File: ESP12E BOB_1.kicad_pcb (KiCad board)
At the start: 2 copper layers, 39.1 x 54.9 mm, 24 parts, among them M1 ESP-12E, P1 CONN_01X07, P2 CONN_01X13, P3 CONN_01X13, P4 CONN_01X01, P5 CONN_01X01, P6 CONN_01X01, P7 CONN_01X01, Q1 BSS138, Q2 BSS138, SW1 SW_PUSH, U1 1117-3.3

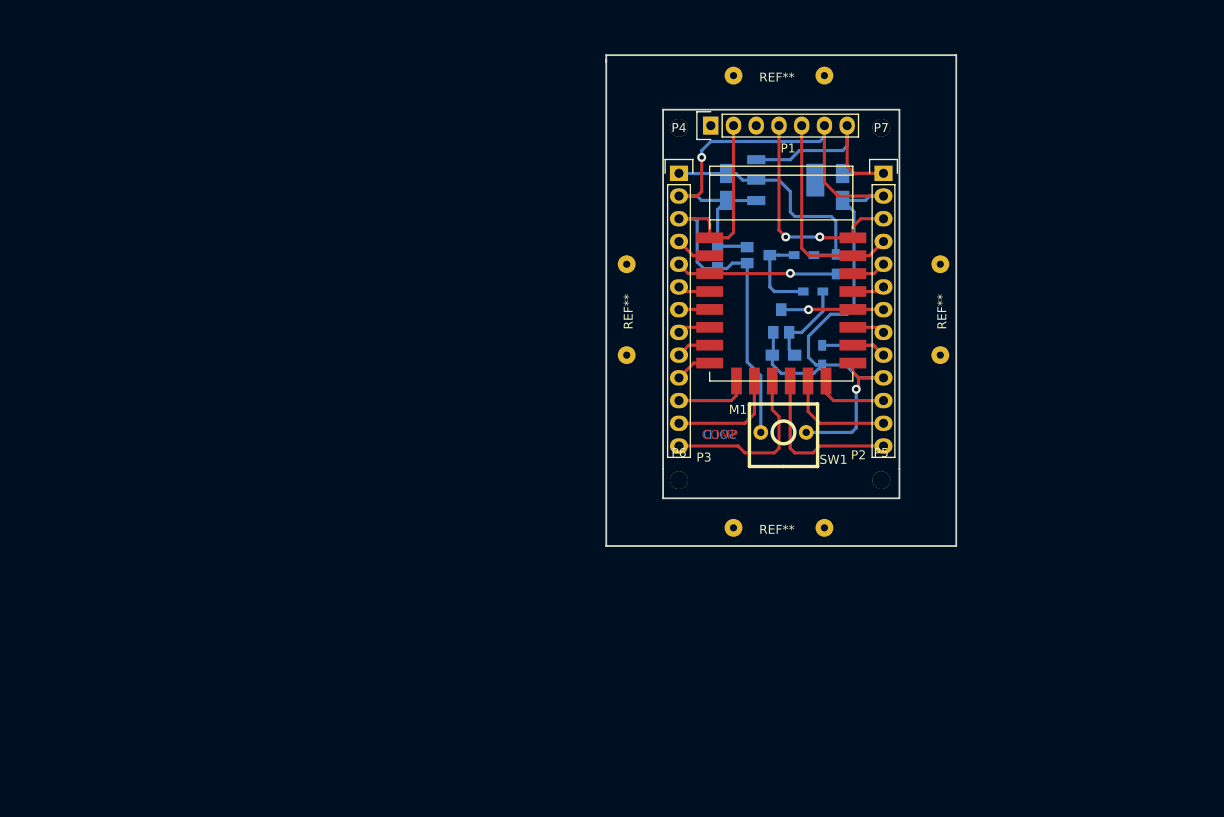
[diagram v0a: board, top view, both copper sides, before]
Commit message: ADDED FILES
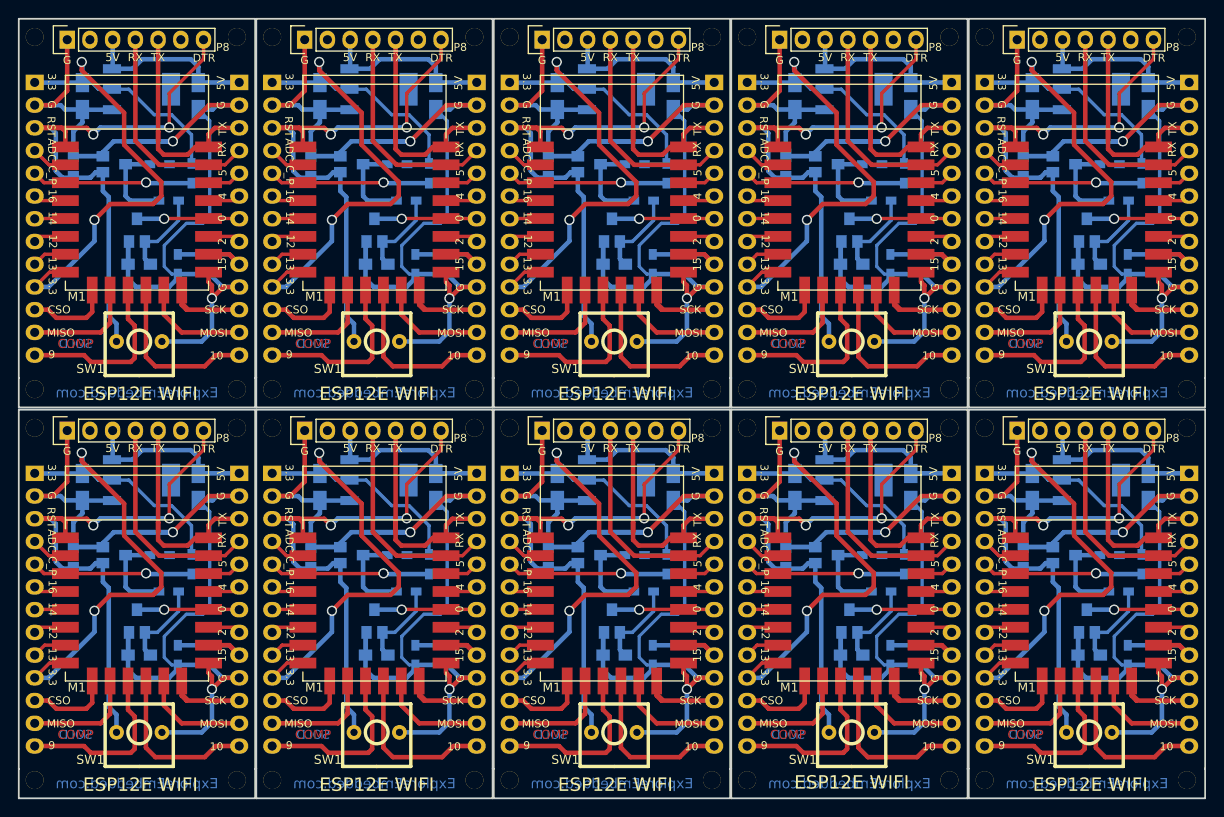
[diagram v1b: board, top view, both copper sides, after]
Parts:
- removed P1: CONN_01X07, Pin_Headers:Pin_Header_Straight_1x07
- removed the P2 at (137.2, 48.3)
- removed REF** (x4): WireConnection_0-8mmDrill, Wire_Connections_Bridges:WireConnection_0-8mmDrill
- added C1: 0.1u, Capacitors_SMD:C_0805_HandSoldering, B.Cu at (152.8, 91.2)
- added C1: 0.1u, Capacitors_SMD:C_0805_HandSoldering, B.Cu at (126.2, 91.2)
- added C1: 0.1u, Capacitors_SMD:C_0805_HandSoldering, B.Cu at (99.7, 91.2)
- added C1: 0.1u, Capacitors_SMD:C_0805_HandSoldering, B.Cu at (73.2, 91.2)
- added C1: 0.1u, Capacitors_SMD:C_0805_HandSoldering, B.Cu at (46.6, 91.2)
- added C1: 0.1u, Capacitors_SMD:C_0805_HandSoldering, B.Cu at (152.8, 47.5)
- added C1: 0.1u, Capacitors_SMD:C_0805_HandSoldering, B.Cu at (126.2, 47.5)
- added C1: 0.1u, Capacitors_SMD:C_0805_HandSoldering, B.Cu at (99.7, 47.5)
- added C1: 0.1u, Capacitors_SMD:C_0805_HandSoldering, B.Cu at (73.2, 47.5)
- added C2: 2u2, Capacitors_SMD:C_0805_HandSoldering, B.Cu at (160.1, 102.1)
- added C2: 2u2, Capacitors_SMD:C_0805_HandSoldering, B.Cu at (133.6, 102.1)
- added C2: 2u2, Capacitors_SMD:C_0805_HandSoldering, B.Cu at (107.1, 102.1)
- added C2: 2u2, Capacitors_SMD:C_0805_HandSoldering, B.Cu at (80.5, 102.1)
- added C2: 2u2, Capacitors_SMD:C_0805_HandSoldering, B.Cu at (54.0, 102.1)
- added C2: 2u2, Capacitors_SMD:C_0805_HandSoldering, B.Cu at (160.1, 58.4)
- added C2: 2u2, Capacitors_SMD:C_0805_HandSoldering, B.Cu at (133.6, 58.4)
- added C2: 2u2, Capacitors_SMD:C_0805_HandSoldering, B.Cu at (107.1, 58.4)
- added C2: 2u2, Capacitors_SMD:C_0805_HandSoldering, B.Cu at (80.5, 58.4)
- added C3: 4u7, Capacitors_Tantalum_SMD:TantalC_SizeA_EIA-3216_Wave, B.Cu at (166.8, 83.3)
- added C3: 4u7, Capacitors_Tantalum_SMD:TantalC_SizeA_EIA-3216_Wave, B.Cu at (140.2, 83.3)
- added C3: 4u7, Capacitors_Tantalum_SMD:TantalC_SizeA_EIA-3216_Wave, B.Cu at (113.7, 83.3)
- added C3: 4u7, Capacitors_Tantalum_SMD:TantalC_SizeA_EIA-3216_Wave, B.Cu at (87.1, 83.3)
- added C3: 4u7, Capacitors_Tantalum_SMD:TantalC_SizeA_EIA-3216_Wave, B.Cu at (60.6, 83.3)
- added C3: 4u7, Capacitors_Tantalum_SMD:TantalC_SizeA_EIA-3216_Wave, B.Cu at (166.8, 39.6)
- added C3: 4u7, Capacitors_Tantalum_SMD:TantalC_SizeA_EIA-3216_Wave, B.Cu at (140.2, 39.6)
- added C3: 4u7, Capacitors_Tantalum_SMD:TantalC_SizeA_EIA-3216_Wave, B.Cu at (113.7, 39.6)
- added C3: 4u7, Capacitors_Tantalum_SMD:TantalC_SizeA_EIA-3216_Wave, B.Cu at (87.1, 39.6)
- added C4: 10u, Capacitors_Tantalum_SMD:TantalC_SizeA_EIA-3216_Wave, B.Cu at (153.8, 83.3)
- added C4: 10u, Capacitors_Tantalum_SMD:TantalC_SizeA_EIA-3216_Wave, B.Cu at (127.3, 83.3)
- added C4: 10u, Capacitors_Tantalum_SMD:TantalC_SizeA_EIA-3216_Wave, B.Cu at (100.7, 83.3)
- added C4: 10u, Capacitors_Tantalum_SMD:TantalC_SizeA_EIA-3216_Wave, B.Cu at (74.2, 83.3)
- added C4: 10u, Capacitors_Tantalum_SMD:TantalC_SizeA_EIA-3216_Wave, B.Cu at (47.6, 83.3)
- added C4: 10u, Capacitors_Tantalum_SMD:TantalC_SizeA_EIA-3216_Wave, B.Cu at (153.8, 39.6)
- added C4: 10u, Capacitors_Tantalum_SMD:TantalC_SizeA_EIA-3216_Wave, B.Cu at (127.3, 39.6)
- added C4: 10u, Capacitors_Tantalum_SMD:TantalC_SizeA_EIA-3216_Wave, B.Cu at (100.7, 39.6)
- added C4: 10u, Capacitors_Tantalum_SMD:TantalC_SizeA_EIA-3216_Wave, B.Cu at (74.2, 39.6)
- added M1: ESP-12E, ESP12E:ESP-12E, F.Cu at (159.9, 95.0)
- added M1: ESP-12E, ESP12E:ESP-12E, F.Cu at (133.3, 95.0)
- added M1: ESP-12E, ESP12E:ESP-12E, F.Cu at (106.8, 95.0)
- added M1: ESP-12E, ESP12E:ESP-12E, F.Cu at (80.3, 95.0)
- added M1: ESP-12E, ESP12E:ESP-12E, F.Cu at (53.7, 95.0)
- added M1: ESP-12E, ESP12E:ESP-12E, F.Cu at (159.9, 51.3)
- added M1: ESP-12E, ESP12E:ESP-12E, F.Cu at (133.3, 51.3)
- added M1: ESP-12E, ESP12E:ESP-12E, F.Cu at (106.8, 51.3)
- added M1: ESP-12E, ESP12E:ESP-12E, F.Cu at (80.3, 51.3)
- added P2: CONN_01X13, Pin_Headers:Pin_Header_Straight_1x13, B.Cu at (171.3, 81.8)
- added P2: CONN_01X13, Pin_Headers:Pin_Header_Straight_1x13, B.Cu at (65.2, 38.1)
- added P2: CONN_01X13, Pin_Headers:Pin_Header_Straight_1x13, B.Cu at (144.8, 81.8)
- added P2: CONN_01X13, Pin_Headers:Pin_Header_Straight_1x13, B.Cu at (118.2, 81.8)
- added P2: CONN_01X13, Pin_Headers:Pin_Header_Straight_1x13, B.Cu at (91.7, 81.8)
- added P2: CONN_01X13, Pin_Headers:Pin_Header_Straight_1x13, B.Cu at (65.2, 81.8)
- added P2: CONN_01X13, Pin_Headers:Pin_Header_Straight_1x13, B.Cu at (171.3, 38.1)
- added P2: CONN_01X13, Pin_Headers:Pin_Header_Straight_1x13, B.Cu at (144.8, 38.1)
- added P2: CONN_01X13, Pin_Headers:Pin_Header_Straight_1x13, B.Cu at (118.2, 38.1)
- added P2: CONN_01X13, Pin_Headers:Pin_Header_Straight_1x13, B.Cu at (91.7, 38.1)
- added P3: CONN_01X13, Pin_Headers:Pin_Header_Straight_1x13, B.Cu at (148.5, 81.8)
- added P3: CONN_01X13, Pin_Headers:Pin_Header_Straight_1x13, B.Cu at (121.9, 81.8)
- added P3: CONN_01X13, Pin_Headers:Pin_Header_Straight_1x13, B.Cu at (95.4, 81.8)
- added P3: CONN_01X13, Pin_Headers:Pin_Header_Straight_1x13, B.Cu at (68.8, 81.8)
- added P3: CONN_01X13, Pin_Headers:Pin_Header_Straight_1x13, B.Cu at (42.3, 81.8)
- added P3: CONN_01X13, Pin_Headers:Pin_Header_Straight_1x13, B.Cu at (148.5, 38.1)
- added P3: CONN_01X13, Pin_Headers:Pin_Header_Straight_1x13, B.Cu at (121.9, 38.1)
- added P3: CONN_01X13, Pin_Headers:Pin_Header_Straight_1x13, B.Cu at (95.4, 38.1)
- added P3: CONN_01X13, Pin_Headers:Pin_Header_Straight_1x13, B.Cu at (68.8, 38.1)
- added P4: CONN_01X01, Connect:1pin, F.Cu at (148.5, 76.7)
- added P4: CONN_01X01, Connect:1pin, F.Cu at (121.9, 76.7)
- added P4: CONN_01X01, Connect:1pin, F.Cu at (95.4, 76.7)
- added P4: CONN_01X01, Connect:1pin, F.Cu at (68.8, 76.7)
- added P4: CONN_01X01, Connect:1pin, F.Cu at (42.3, 76.7)
- added P4: CONN_01X01, Connect:1pin, F.Cu at (148.5, 33.0)
- added P4: CONN_01X01, Connect:1pin, F.Cu at (121.9, 33.0)
- added P4: CONN_01X01, Connect:1pin, F.Cu at (95.4, 33.0)
- added P4: CONN_01X01, Connect:1pin, F.Cu at (68.8, 33.0)
- added P5: CONN_01X01, Connect:1pin, F.Cu at (171.1, 116.1)
- added P5: CONN_01X01, Connect:1pin, F.Cu at (144.5, 116.1)
- added P5: CONN_01X01, Connect:1pin, F.Cu at (118.0, 116.1)
- added P5: CONN_01X01, Connect:1pin, F.Cu at (91.4, 116.1)
- added P5: CONN_01X01, Connect:1pin, F.Cu at (64.9, 116.1)
- added P5: CONN_01X01, Connect:1pin, F.Cu at (171.1, 72.4)
- added P5: CONN_01X01, Connect:1pin, F.Cu at (144.5, 72.4)
- added P5: CONN_01X01, Connect:1pin, F.Cu at (118.0, 72.4)
- added P5: CONN_01X01, Connect:1pin, F.Cu at (91.4, 72.4)
- added P6: CONN_01X01, Connect:1pin, F.Cu at (148.5, 116.1)
- added P6: CONN_01X01, Connect:1pin, F.Cu at (121.9, 116.1)
- added P6: CONN_01X01, Connect:1pin, F.Cu at (95.4, 116.1)
- added P6: CONN_01X01, Connect:1pin, F.Cu at (68.8, 116.1)
- added P6: CONN_01X01, Connect:1pin, F.Cu at (42.3, 116.1)
- added P6: CONN_01X01, Connect:1pin, F.Cu at (148.5, 72.4)
- added P6: CONN_01X01, Connect:1pin, F.Cu at (121.9, 72.4)
- added P6: CONN_01X01, Connect:1pin, F.Cu at (95.4, 72.4)
- added P6: CONN_01X01, Connect:1pin, F.Cu at (68.8, 72.4)
- added P7: CONN_01X01, Connect:1pin, F.Cu at (171.1, 76.7)
- added P7: CONN_01X01, Connect:1pin, F.Cu at (144.5, 76.7)
- added P7: CONN_01X01, Connect:1pin, F.Cu at (118.0, 76.7)
- added P7: CONN_01X01, Connect:1pin, F.Cu at (91.4, 76.7)
- added P7: CONN_01X01, Connect:1pin, F.Cu at (64.9, 76.7)
- added P7: CONN_01X01, Connect:1pin, F.Cu at (171.1, 33.0)
- added P7: CONN_01X01, Connect:1pin, F.Cu at (144.5, 33.0)
- added P7: CONN_01X01, Connect:1pin, F.Cu at (118.0, 33.0)
- added P7: CONN_01X01, Connect:1pin, F.Cu at (91.4, 33.0)
- added P8: CONN_01X07, Pin_Headers:Pin_Header_Straight_1x07, F.Cu at (152.1, 77.0)
- added P8: CONN_01X07, Pin_Headers:Pin_Header_Straight_1x07, F.Cu at (45.9, 33.3)
- added P8: CONN_01X07, Pin_Headers:Pin_Header_Straight_1x07, F.Cu at (125.6, 77.0)
- added P8: CONN_01X07, Pin_Headers:Pin_Header_Straight_1x07, F.Cu at (99.0, 77.0)
- added P8: CONN_01X07, Pin_Headers:Pin_Header_Straight_1x07, F.Cu at (72.5, 77.0)
- added P8: CONN_01X07, Pin_Headers:Pin_Header_Straight_1x07, F.Cu at (45.9, 77.0)
- added P8: CONN_01X07, Pin_Headers:Pin_Header_Straight_1x07, F.Cu at (152.1, 33.3)
- added P8: CONN_01X07, Pin_Headers:Pin_Header_Straight_1x07, F.Cu at (125.6, 33.3)
- added P8: CONN_01X07, Pin_Headers:Pin_Header_Straight_1x07, F.Cu at (99.0, 33.3)
- added P8: CONN_01X07, Pin_Headers:Pin_Header_Straight_1x07, F.Cu at (72.5, 33.3)
- added Q1: BSS138, ESP12E:SOT-23-GDS, B.Cu at (157.4, 90.9)
- added Q1: BSS138, ESP12E:SOT-23-GDS, B.Cu at (130.8, 90.9)
- added Q1: BSS138, ESP12E:SOT-23-GDS, B.Cu at (104.3, 90.9)
- added Q1: BSS138, ESP12E:SOT-23-GDS, B.Cu at (77.7, 90.9)
- added Q1: BSS138, ESP12E:SOT-23-GDS, B.Cu at (51.2, 90.9)
- added Q1: BSS138, ESP12E:SOT-23-GDS, B.Cu at (157.4, 47.2)
- added Q1: BSS138, ESP12E:SOT-23-GDS, B.Cu at (130.8, 47.2)
- added Q1: BSS138, ESP12E:SOT-23-GDS, B.Cu at (104.3, 47.2)
- added Q1: BSS138, ESP12E:SOT-23-GDS, B.Cu at (77.7, 47.2)
- added Q2: BSS138, ESP12E:SOT-23-GDS, B.Cu at (159.9, 98.3)
- added Q2: BSS138, ESP12E:SOT-23-GDS, B.Cu at (133.3, 98.3)
- added Q2: BSS138, ESP12E:SOT-23-GDS, B.Cu at (106.8, 98.3)
- added Q2: BSS138, ESP12E:SOT-23-GDS, B.Cu at (80.3, 98.3)
- added Q2: BSS138, ESP12E:SOT-23-GDS, B.Cu at (53.7, 98.3)
- added Q2: BSS138, ESP12E:SOT-23-GDS, B.Cu at (159.9, 54.6)
- added Q2: BSS138, ESP12E:SOT-23-GDS, B.Cu at (133.3, 54.6)
- added Q2: BSS138, ESP12E:SOT-23-GDS, B.Cu at (106.8, 54.6)
- added Q2: BSS138, ESP12E:SOT-23-GDS, B.Cu at (80.3, 54.6)
- added R1: 470K, Resistors_SMD:R_0603_HandSoldering, B.Cu at (162.4, 90.9)
- added R1: 470K, Resistors_SMD:R_0603_HandSoldering, B.Cu at (135.9, 90.9)
- added R1: 470K, Resistors_SMD:R_0603_HandSoldering, B.Cu at (109.3, 90.9)
- added R1: 470K, Resistors_SMD:R_0603_HandSoldering, B.Cu at (82.8, 90.9)
- added R1: 470K, Resistors_SMD:R_0603_HandSoldering, B.Cu at (56.3, 90.9)
- added R1: 470K, Resistors_SMD:R_0603_HandSoldering, B.Cu at (162.4, 47.2)
- added R1: 470K, Resistors_SMD:R_0603_HandSoldering, B.Cu at (135.9, 47.2)
- added R1: 470K, Resistors_SMD:R_0603_HandSoldering, B.Cu at (109.3, 47.2)
- added R1: 470K, Resistors_SMD:R_0603_HandSoldering, B.Cu at (82.8, 47.2)
- added R2: 100K, Resistors_SMD:R_0603_HandSoldering, B.Cu at (163.4, 95.0)
- added R2: 100K, Resistors_SMD:R_0603_HandSoldering, B.Cu at (136.9, 95.0)
- added R2: 100K, Resistors_SMD:R_0603_HandSoldering, B.Cu at (110.4, 95.0)
- added R2: 100K, Resistors_SMD:R_0603_HandSoldering, B.Cu at (83.8, 95.0)
- added R2: 100K, Resistors_SMD:R_0603_HandSoldering, B.Cu at (57.3, 95.0)
- added R2: 100K, Resistors_SMD:R_0603_HandSoldering, B.Cu at (163.4, 51.3)
- added R2: 100K, Resistors_SMD:R_0603_HandSoldering, B.Cu at (136.9, 51.3)
- added R2: 100K, Resistors_SMD:R_0603_HandSoldering, B.Cu at (110.4, 51.3)
- added R2: 100K, Resistors_SMD:R_0603_HandSoldering, B.Cu at (83.8, 51.3)
- added R3: 10K, Resistors_SMD:R_0603_HandSoldering, B.Cu at (164.5, 102.1)
- added R3: 10K, Resistors_SMD:R_0603_HandSoldering, B.Cu at (137.9, 102.1)
- added R3: 10K, Resistors_SMD:R_0603_HandSoldering, B.Cu at (111.4, 102.1)
- added R3: 10K, Resistors_SMD:R_0603_HandSoldering, B.Cu at (84.8, 102.1)
- added R3: 10K, Resistors_SMD:R_0603_HandSoldering, B.Cu at (58.3, 102.1)
- added R3: 10K, Resistors_SMD:R_0603_HandSoldering, B.Cu at (164.5, 58.4)
- added R3: 10K, Resistors_SMD:R_0603_HandSoldering, B.Cu at (137.9, 58.4)
- added R3: 10K, Resistors_SMD:R_0603_HandSoldering, B.Cu at (111.4, 58.4)
- added R3: 10K, Resistors_SMD:R_0603_HandSoldering, B.Cu at (84.8, 58.4)
- added R4: 47K, Resistors_SMD:R_0603_HandSoldering, B.Cu at (166.0, 91.9)
- added R4: 47K, Resistors_SMD:R_0603_HandSoldering, B.Cu at (139.4, 91.9)
- added R4: 47K, Resistors_SMD:R_0603_HandSoldering, B.Cu at (112.9, 91.9)
- added R4: 47K, Resistors_SMD:R_0603_HandSoldering, B.Cu at (86.4, 91.9)
- added R4: 47K, Resistors_SMD:R_0603_HandSoldering, B.Cu at (59.8, 91.9)
- added R4: 47K, Resistors_SMD:R_0603_HandSoldering, B.Cu at (166.0, 48.3)
- added R4: 47K, Resistors_SMD:R_0603_HandSoldering, B.Cu at (139.4, 48.3)
- added R4: 47K, Resistors_SMD:R_0603_HandSoldering, B.Cu at (112.9, 48.3)
- added R4: 47K, Resistors_SMD:R_0603_HandSoldering, B.Cu at (86.4, 48.3)
- added SW1: SW_PUSH, ESP12E:SW_PUSH_SMALL_2pin_xl, F.Cu at (160.1, 110.7)
- added SW1: SW_PUSH, ESP12E:SW_PUSH_SMALL_2pin_xl, F.Cu at (133.6, 110.7)
- added SW1: SW_PUSH, ESP12E:SW_PUSH_SMALL_2pin_xl, F.Cu at (107.1, 110.7)
- added SW1: SW_PUSH, ESP12E:SW_PUSH_SMALL_2pin_xl, F.Cu at (80.5, 110.7)
- added SW1: SW_PUSH, ESP12E:SW_PUSH_SMALL_2pin_xl, F.Cu at (54.0, 110.7)
- added SW1: SW_PUSH, ESP12E:SW_PUSH_SMALL_2pin_xl, F.Cu at (160.1, 67.1)
- added SW1: SW_PUSH, ESP12E:SW_PUSH_SMALL_2pin_xl, F.Cu at (133.6, 67.1)
- added SW1: SW_PUSH, ESP12E:SW_PUSH_SMALL_2pin_xl, F.Cu at (107.1, 67.1)
- added SW1: SW_PUSH, ESP12E:SW_PUSH_SMALL_2pin_xl, F.Cu at (80.5, 67.1)
- added U1: 1117-3.3, SMD_Packages:SOT-223, B.Cu at (160.4, 82.5)
- added U1: 1117-3.3, SMD_Packages:SOT-223, B.Cu at (133.9, 82.5)
- added U1: 1117-3.3, SMD_Packages:SOT-223, B.Cu at (107.3, 82.5)
- added U1: 1117-3.3, SMD_Packages:SOT-223, B.Cu at (80.8, 82.5)
- added U1: 1117-3.3, SMD_Packages:SOT-223, B.Cu at (54.2, 82.5)
- added U1: 1117-3.3, SMD_Packages:SOT-223, B.Cu at (160.4, 38.9)
- added U1: 1117-3.3, SMD_Packages:SOT-223, B.Cu at (133.9, 38.9)
- added U1: 1117-3.3, SMD_Packages:SOT-223, B.Cu at (107.3, 38.9)
- added U1: 1117-3.3, SMD_Packages:SOT-223, B.Cu at (80.8, 38.9)
- P3: moved to B.Cu
- moved M1 72.7 mm to (53.7, 51.3)
- moved Q2 72.7 mm to (53.7, 54.6)
- moved R1 72.7 mm to (56.3, 47.2)
- moved C4 72.7 mm to (47.6, 39.6)
- moved P3 72.7 mm to (42.3, 38.1), turned to 180 degrees
- moved P4 72.7 mm to (42.3, 33.0)
- moved P5 72.7 mm to (64.9, 72.4)
- moved P6 72.7 mm to (42.3, 72.4)
- moved P7 72.7 mm to (64.9, 33.0)
- moved Q1 72.7 mm to (51.2, 47.2)
- moved R2 72.7 mm to (57.3, 51.3)
- moved U1 72.7 mm to (54.2, 38.9)
- moved C1 72.7 mm to (46.6, 47.5)
- moved C2 72.7 mm to (54.0, 58.4)
- moved C3 72.7 mm to (60.6, 39.6)
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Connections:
- M1 pad 21: /TX -> /RX
- M1 pad 22: /RX -> /TX
- M1 pad 8: Net-(M1-Pad8) -> +3V3
- P3 pad 10: Net-(M1-Pad8) -> +3V3
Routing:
- net GND: track 115.8 -> 1203.7 mm, vias 2 -> 20
- net +3V3: track 27.3 -> 705.4 mm, vias 0 -> 20
- net /DTR: track 54.0 -> 676.8 mm, vias 0 -> 20
- net Net-(M1-Pad11): track 19.5 -> 282.1 mm
- net /TX: track 23.9 -> 246.9 mm
- net /RX: track 25.3 -> 246.9 mm, vias 2 -> 0
- net +5V: track 26.6 -> 246.6 mm
- net Net-(M1-Pad10): track 12.5 -> 214.1 mm
- net Net-(M1-Pad3): track 18.0 -> 196.1 mm, vias 1 -> 10
- net /GPIO10: track 18.5 -> 188.4 mm
- net /SCK: track 8.13 -> 164.4 mm
- net Net-(Q1-PadD): track 10.2 -> 144.8 mm
- net Net-(M1-Pad16): track 11.2 -> 127.8 mm
- net /MOSI: track 12.4 -> 119.9 mm
- net /GPIO0: track 11.5 -> 115.0 mm, vias 1 -> 10
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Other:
- board size 39.1 x 54.9 mm -> 132.6 x 87.1 mm
- net class Default: clearance 0.5 -> 0.1778
- rule trace_clearance: 0.5 -> 0.1778
- board text added: "0"
- board text added: "10"
- board text added: "12"
- board text added: "13"
- board text added: "14"
- board text added: "15"
- board text added: "16"
- board text added: "2"
- board text added: "3.3"
- board text added: "4"
- board text added: "5"
- board text added: "5V"
- board text added: "9"
- board text added: "ADC"
- board text added: "CSO"
- board text added: "C_P"
- board text added: "DTR"
- board text added: "ESP12E WIFI"
- board text added: "ExploreEmbedded.com"
- board text added: "G"
- board text added: "MISO"
- board text added: "MOSI"
- board text added: "RST"
- board text added: "RX"
- board text added: "SCK"
- board text added: "TX"
- board text removed: "1. module 3.3V no connected. 2. UART connections 3. Keep board mounting holes 2mm. 4. Labels should be reflect on the baord."

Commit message: ADDED NEW FILES
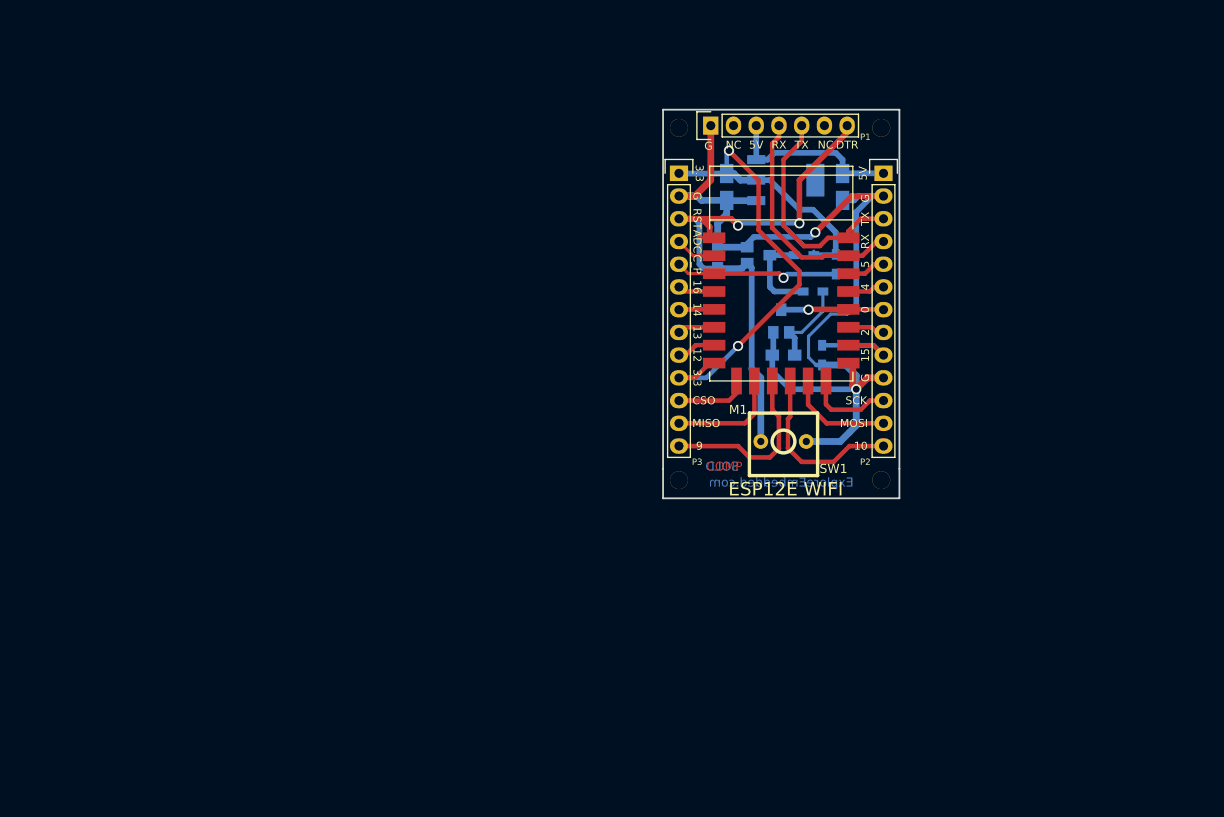
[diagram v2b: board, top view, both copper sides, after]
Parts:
- removed the C1 at (152.8, 91.2)
- removed the C1 at (126.2, 91.2)
- removed the C1 at (99.7, 91.2)
- removed the C1 at (73.2, 91.2)
- removed the C1 at (46.6, 91.2)
- removed the C1 at (152.8, 47.5)
- removed the C1 at (126.2, 47.5)
- removed the C1 at (99.7, 47.5)
- removed the C1 at (73.2, 47.5)
- removed the C2 at (160.1, 102.1)
- removed the C2 at (133.6, 102.1)
- removed the C2 at (107.1, 102.1)
- removed the C2 at (80.5, 102.1)
- removed the C2 at (54.0, 102.1)
- removed the C2 at (160.1, 58.4)
- removed the C2 at (133.6, 58.4)
- removed the C2 at (107.1, 58.4)
- removed the C2 at (80.5, 58.4)
- removed the C3 at (166.8, 83.3)
- removed the C3 at (60.6, 39.6)
- removed the C3 at (140.2, 83.3)
- removed the C3 at (113.7, 83.3)
- removed the C3 at (87.1, 83.3)
- removed the C3 at (60.6, 83.3)
- removed the C3 at (166.8, 39.6)
- removed the C3 at (140.2, 39.6)
- removed the C3 at (113.7, 39.6)
- removed the C3 at (87.1, 39.6)
- removed the C4 at (153.8, 83.3)
- removed the C4 at (127.3, 83.3)
- removed the C4 at (100.7, 83.3)
- removed the C4 at (74.2, 83.3)
- removed the C4 at (47.6, 83.3)
- removed the C4 at (153.8, 39.6)
- removed the C4 at (127.3, 39.6)
- removed the C4 at (100.7, 39.6)
- removed the C4 at (74.2, 39.6)
- removed the M1 at (159.9, 95.0)
- removed the M1 at (133.3, 95.0)
- removed the M1 at (106.8, 95.0)
- removed the M1 at (80.3, 95.0)
- removed the M1 at (53.7, 95.0)
- removed the M1 at (159.9, 51.3)
- removed the M1 at (133.3, 51.3)
- removed the M1 at (106.8, 51.3)
- removed the M1 at (80.3, 51.3)
- removed the P2 at (171.3, 81.8)
- removed the P2 at (65.2, 38.1)
- removed the P2 at (144.8, 81.8)
- removed the P2 at (118.2, 81.8)
- removed the P2 at (91.7, 81.8)
- removed the P2 at (65.2, 81.8)
- removed the P2 at (171.3, 38.1)
- removed the P2 at (144.8, 38.1)
- removed the P2 at (118.2, 38.1)
- removed the P2 at (91.7, 38.1)
- removed the P3 at (148.5, 81.8)
- removed the P3 at (121.9, 81.8)
- removed the P3 at (95.4, 81.8)
- removed the P3 at (68.8, 81.8)
- removed the P3 at (42.3, 81.8)
- removed the P3 at (148.5, 38.1)
- removed the P3 at (121.9, 38.1)
- removed the P3 at (95.4, 38.1)
- removed the P3 at (68.8, 38.1)
- removed the P4 at (148.5, 76.7)
- removed the P4 at (121.9, 76.7)
- removed the P4 at (95.4, 76.7)
- removed the P4 at (68.8, 76.7)
- removed the P4 at (42.3, 76.7)
- removed the P4 at (148.5, 33.0)
- removed the P4 at (121.9, 33.0)
- removed the P4 at (95.4, 33.0)
- removed the P4 at (68.8, 33.0)
- removed the P5 at (171.1, 116.1)
- removed the P5 at (144.5, 116.1)
- removed the P5 at (118.0, 116.1)
- removed the P5 at (91.4, 116.1)
- removed the P5 at (64.9, 116.1)
- removed the P5 at (171.1, 72.4)
- removed the P5 at (144.5, 72.4)
- removed the P5 at (118.0, 72.4)
- removed the P5 at (91.4, 72.4)
- removed the P6 at (148.5, 116.1)
- removed the P6 at (121.9, 116.1)
- removed the P6 at (95.4, 116.1)
- removed the P6 at (68.8, 116.1)
- removed the P6 at (42.3, 116.1)
- removed the P6 at (148.5, 72.4)
- removed the P6 at (121.9, 72.4)
- removed the P6 at (95.4, 72.4)
- removed the P6 at (68.8, 72.4)
- removed the P7 at (171.1, 76.7)
- removed the P7 at (144.5, 76.7)
- removed the P7 at (118.0, 76.7)
- removed the P7 at (91.4, 76.7)
- removed the P7 at (64.9, 76.7)
- removed the P7 at (171.1, 33.0)
- removed the P7 at (144.5, 33.0)
- removed the P7 at (118.0, 33.0)
- removed the P7 at (91.4, 33.0)
- removed P8 (x10): CONN_01X07, Pin_Headers:Pin_Header_Straight_1x07
- removed the Q1 at (157.4, 90.9)
- removed the Q1 at (130.8, 90.9)
- removed the Q1 at (104.3, 90.9)
- removed the Q1 at (77.7, 90.9)
- removed the Q1 at (51.2, 90.9)
- removed the Q1 at (157.4, 47.2)
- removed the Q1 at (130.8, 47.2)
- removed the Q1 at (104.3, 47.2)
- removed the Q1 at (77.7, 47.2)
- removed the Q2 at (159.9, 98.3)
- removed the Q2 at (133.3, 98.3)
- removed the Q2 at (106.8, 98.3)
- removed the Q2 at (80.3, 98.3)
- removed the Q2 at (53.7, 98.3)
- removed the Q2 at (159.9, 54.6)
- removed the Q2 at (133.3, 54.6)
- removed the Q2 at (106.8, 54.6)
- removed the Q2 at (80.3, 54.6)
- removed the R1 at (162.4, 90.9)
- removed the R1 at (135.9, 90.9)
- removed the R1 at (109.3, 90.9)
- removed the R1 at (82.8, 90.9)
- removed the R1 at (56.3, 90.9)
- removed the R1 at (162.4, 47.2)
- removed the R1 at (135.9, 47.2)
- removed the R1 at (109.3, 47.2)
- removed the R1 at (82.8, 47.2)
- removed the R2 at (163.4, 95.0)
- removed the R2 at (136.9, 95.0)
- removed the R2 at (110.4, 95.0)
- removed the R2 at (83.8, 95.0)
- removed the R2 at (57.3, 95.0)
- removed the R2 at (163.4, 51.3)
- removed the R2 at (136.9, 51.3)
- removed the R2 at (110.4, 51.3)
- removed the R2 at (83.8, 51.3)
- removed the R3 at (164.5, 102.1)
- removed the R3 at (137.9, 102.1)
- removed the R3 at (111.4, 102.1)
- removed the R3 at (84.8, 102.1)
- removed the R3 at (58.3, 102.1)
- removed the R3 at (164.5, 58.4)
- removed the R3 at (137.9, 58.4)
- removed the R3 at (111.4, 58.4)
- removed the R3 at (84.8, 58.4)
- removed the R4 at (166.0, 91.9)
- removed the R4 at (139.4, 91.9)
- removed the R4 at (112.9, 91.9)
- removed the R4 at (86.4, 91.9)
- removed the R4 at (59.8, 91.9)
- removed the R4 at (166.0, 48.3)
- removed the R4 at (139.4, 48.3)
- removed the R4 at (112.9, 48.3)
- removed the R4 at (86.4, 48.3)
- removed the SW1 at (160.1, 110.7)
- removed the SW1 at (133.6, 110.7)
- removed the SW1 at (107.1, 110.7)
- removed the SW1 at (80.5, 110.7)
- removed the SW1 at (54.0, 110.7)
- removed the SW1 at (160.1, 67.1)
- removed the SW1 at (133.6, 67.1)
- removed the SW1 at (107.1, 67.1)
- removed the SW1 at (80.5, 67.1)
- removed the U1 at (160.4, 82.5)
- removed the U1 at (133.9, 82.5)
- removed the U1 at (107.3, 82.5)
- removed the U1 at (80.8, 82.5)
- removed the U1 at (54.2, 82.5)
- removed the U1 at (160.4, 38.9)
- removed the U1 at (133.9, 38.9)
- removed the U1 at (107.3, 38.9)
- removed the U1 at (80.8, 38.9)
- added C3: 4u7, Capacitors_Tantalum_SMD:TantalC_SizeA_EIA-3216_Wave, B.Cu at (132.6, 49.8)
- added LOGO: , logo:LOGO (2), B.Cu at (130.8, 69.6)
- added P1: CONN_01X07, Pin_Headers:Pin_Header_Straight_1x07, F.Cu at (117.9, 42.9)
- added P2: CONN_01X13, Pin_Headers:Pin_Header_Straight_1x13, F.Cu at (137.2, 48.3)
- P3: moved to F.Cu
- moved SW1 72.9 mm to (126.0, 78.2)
- moved M1 72.7 mm to (125.7, 61.5)
- moved Q2 72.7 mm to (125.7, 64.8)
- moved R1 72.7 mm to (128.3, 57.4)
- moved C4 72.7 mm to (119.6, 49.8)
- moved P3 72.7 mm to (114.3, 48.3), turned to 0 degrees
- moved P4 72.7 mm to (114.3, 43.2)
- moved P5 72.7 mm to (136.9, 82.5)
- moved P6 72.7 mm to (114.3, 82.5)
- moved P7 72.7 mm to (136.9, 43.2)
- moved Q1 72.7 mm to (123.2, 57.4)
- moved R2 72.7 mm to (129.3, 61.5)
- moved U1 72.7 mm to (126.2, 49.0)
- moved C1 72.7 mm to (118.6, 57.7)
- moved C2 72.7 mm to (126.0, 68.6)
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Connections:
- net /DTR renamed /RESET
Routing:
- net GND: track 1203.7 -> 123.5 mm, vias 20 -> 2
- net +3V3: track 705.4 -> 70.6 mm, vias 20 -> 2
- net /RESET: track 676.8 -> 73.5 mm, vias 20 -> 2
- net Net-(M1-Pad11): track 282.1 -> 20.0 mm
- net +5V: track 246.6 -> 24.8 mm
- net /RX: track 246.9 -> 28.2 mm
- net /TX: track 246.9 -> 34.9 mm
- net Net-(M1-Pad10): track 214.1 -> 21.4 mm
- net Net-(M1-Pad3): track 196.1 -> 18.3 mm, vias 10 -> 1
- net /GPIO10: track 188.4 -> 19.7 mm
- net /SCK: track 164.4 -> 11.1 mm
- net Net-(Q1-PadD): track 144.8 -> 10.2 mm
- net Net-(M1-Pad16): track 127.8 -> 15.6 mm
- net /MOSI: track 119.9 -> 11.9 mm
- net /GPIO0: track 115.0 -> 15.4 mm, vias 10 -> 1
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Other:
- board size 132.6 x 87.1 mm -> 26.4 x 43.4 mm
- net class Default: clearance 0.1778 -> 0.5
- rule trace_clearance: 0.1778 -> 0.5
- board text added: "NC"
